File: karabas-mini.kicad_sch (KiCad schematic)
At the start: 4 parts

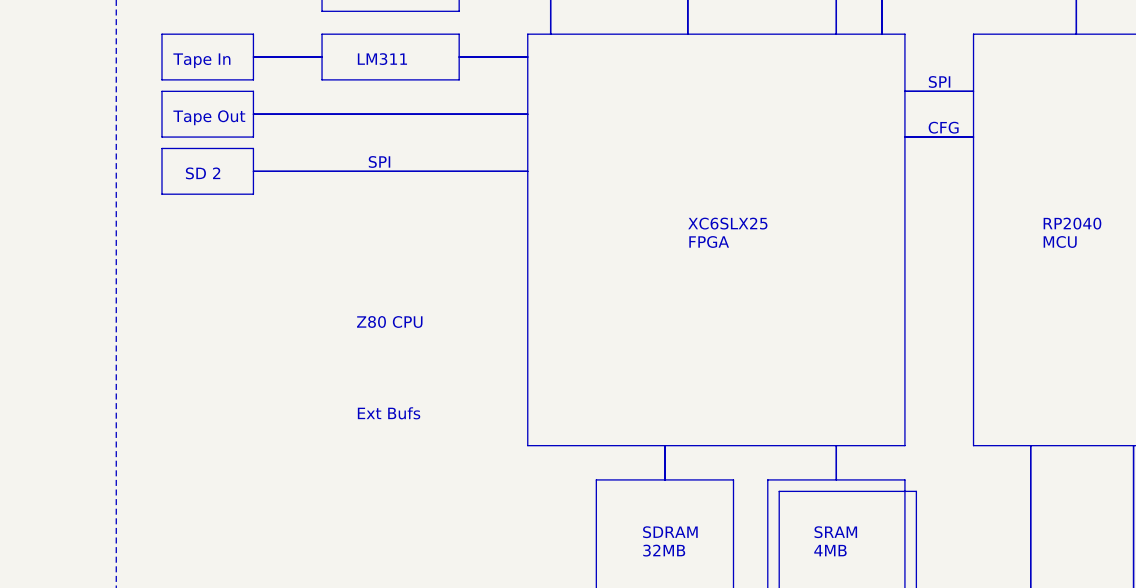
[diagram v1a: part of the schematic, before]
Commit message: Updated revB
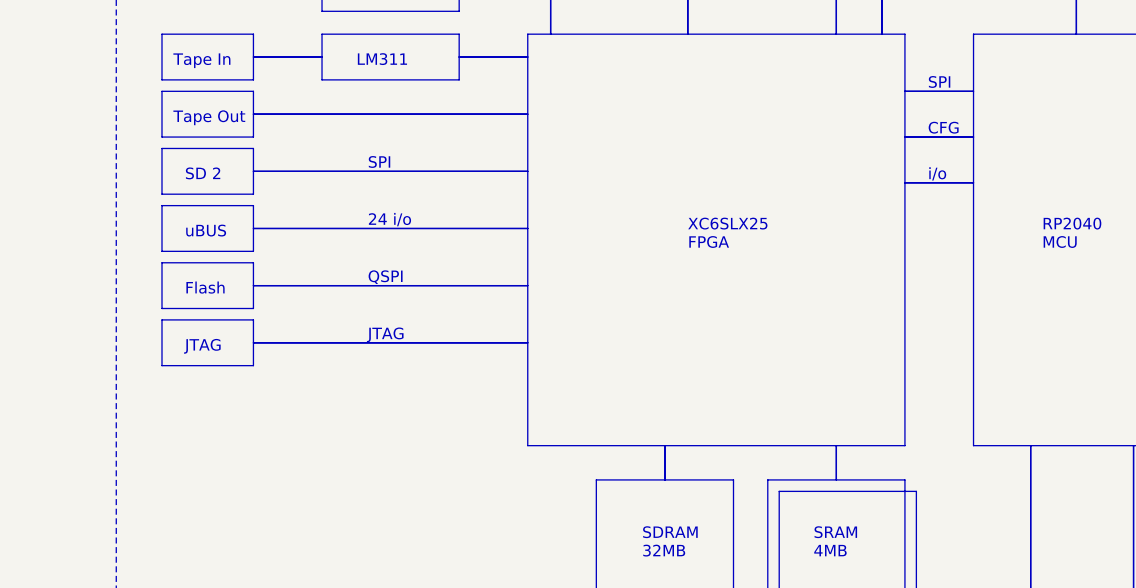
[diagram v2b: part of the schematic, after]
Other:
- note added: "24 i/o"
- note added: "JTAG"
- note added: "i/o"
- note added: "uBUS"
- note removed: "Ext Bufs"
- note removed: "Z80 CPU"
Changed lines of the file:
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@@
   (title_block
     (title "Karabas-Mini")
-    (date "2024-02-20")
-    (rev "A")
+    (date "2024-02-23")
+    (rev "B")
   )
   (rectangle (start 254 132.08) (end 264.16 137.16)
@@
     (fill (type none))
   )
+  (rectangle (start 194.31 91.44) (end 201.93 91.44)
+    (stroke (width 0) (type default))
+    (fill (type none))
+  )
   (rectangle (start 162.56 66.04) (end 177.8 71.12)
     (stroke (width 0) (type default))
@@
     (fill (type none))
   )
+  (rectangle (start 121.92 96.52) (end 152.4 96.52)
+    (stroke (width 0) (type default))
+    (fill (type none))
+  )
   (rectangle (start 144.78 69.85) (end 154.94 69.85)
     (stroke (width 0) (type default))
@@
     (fill (type none))
   )
+  (rectangle (start 111.76 106.68) (end 121.92 111.76)
+    (stroke (width 0) (type default))
+    (fill (type color) (color 255 255 194 1))
+  )
+  (rectangle (start 111.76 100.33) (end 121.92 105.41)
+    (stroke (width 0) (type default))
+    (fill (type color) (color 255 255 194 1))
+  )
   (rectangle (start 208.28 120.65) (end 208.28 138.43)
     (stroke (width 0) (type default))
@@
     (fill (type color) (color 255 255 194 1))
   )
+  (rectangle (start 121.92 102.87) (end 152.4 102.87)
+    (stroke (width 0) (type default))
+    (fill (type none))
+  )
   (rectangle (start 121.92 77.47) (end 129.54 77.47)
     (stroke (width 0) (type default))
@@
     (stroke (width 0) (type default))
     (fill (type none))
+  )
+  (rectangle (start 111.76 93.98) (end 121.92 99.06)
+    (stroke (width 0) (type default))
+    (fill (type color) (color 255 255 194 1))
   )
   (rectangle (start 226.06 81.28) (end 232.41 81.28)
@@
     (fill (type none))
   )
+  (rectangle (start 121.92 109.22) (end 152.4 109.22)
+    (stroke (width 0) (type default))
+    (fill (type none))
+  )
   (rectangle (start 33.02 34.29) (end 87.63 149.86)
     (stroke (width 0) (type dash))
@@
     (effects (font (size 1.27 1.27)) (justify left bottom))
   )
+  (text "24 i/o" (at 134.62 96.52 0)
+    (effects (font (size 1.27 1.27)) (justify left bottom))
+  )
+  (text "Flash" (at 114.3 104.14 0)
+    (effects (font (size 1.27 1.27)) (justify left bottom))
+  )
+  (text "i/o" (at 196.85 91.44 0)
+    (effects (font (size 1.27 1.27)) (justify left bottom))
+  )
   (text "XC6SLX25\nFPGA" (at 170.18 99.06 0)
     (effects (font (size 1.27 1.27)) (justify left bottom))
@@
     (effects (font (size 1.27 1.27)) (justify left bottom))
   )
-  (text "Z80 CPU" (at 133.35 107.95 0)
-    (effects (font (size 1.27 1.27) (color 255 255 255 1)) (justify left bottom))
-  )
   (text "SPI" (at 227.33 115.57 0)
     (effects (font (size 1.27 1.27)) (justify left bottom))
@@
     (effects (font (size 1.27 1.27)) (justify left bottom))
   )
-  (text "Ext Bufs" (at 133.35 118.11 0)
-    (effects (font (size 1.27 1.27) (color 255 255 255 1)) (justify left bottom))
-  )
   (text "SRAM\n4MB" (at 184.15 133.35 0)
     (effects (font (size 1.27 1.27)) (justify left bottom))
@@
     (effects (font (size 1.27 1.27)) (justify left bottom))
   )
+  (text "QSPI" (at 134.62 102.87 0)
+    (effects (font (size 1.27 1.27)) (justify left bottom))
+  )
   (text "Functional schematics" (at 109.22 39.37 0)
     (effects (font (size 1.27 1.27)) (justify left bottom))
@@
     (effects (font (size 1.27 1.27)) (justify left bottom))
   )
+  (text "uBUS" (at 114.3 97.79 0)
+    (effects (font (size 1.27 1.27)) (justify left bottom))
+  )
   (text "CFG" (at 196.85 86.36 0)
     (effects (font (size 1.27 1.27)) (justify left bottom))
@@
     (effects (font (size 1.27 1.27)) (justify left bottom))
   )
+  (text "JTAG" (at 134.62 109.22 0)
+    (effects (font (size 1.27 1.27)) (justify left bottom))
+  )
   (text "USB C" (at 256.54 72.39 0)
     (effects (font (size 1.27 1.27)) (justify left bottom))
@@
     (effects (font (size 1.27 1.27)) (justify left bottom))
   )
+  (text "JTAG" (at 114.3 110.49 0)
+    (effects (font (size 1.27 1.27)) (justify left bottom))
+  )

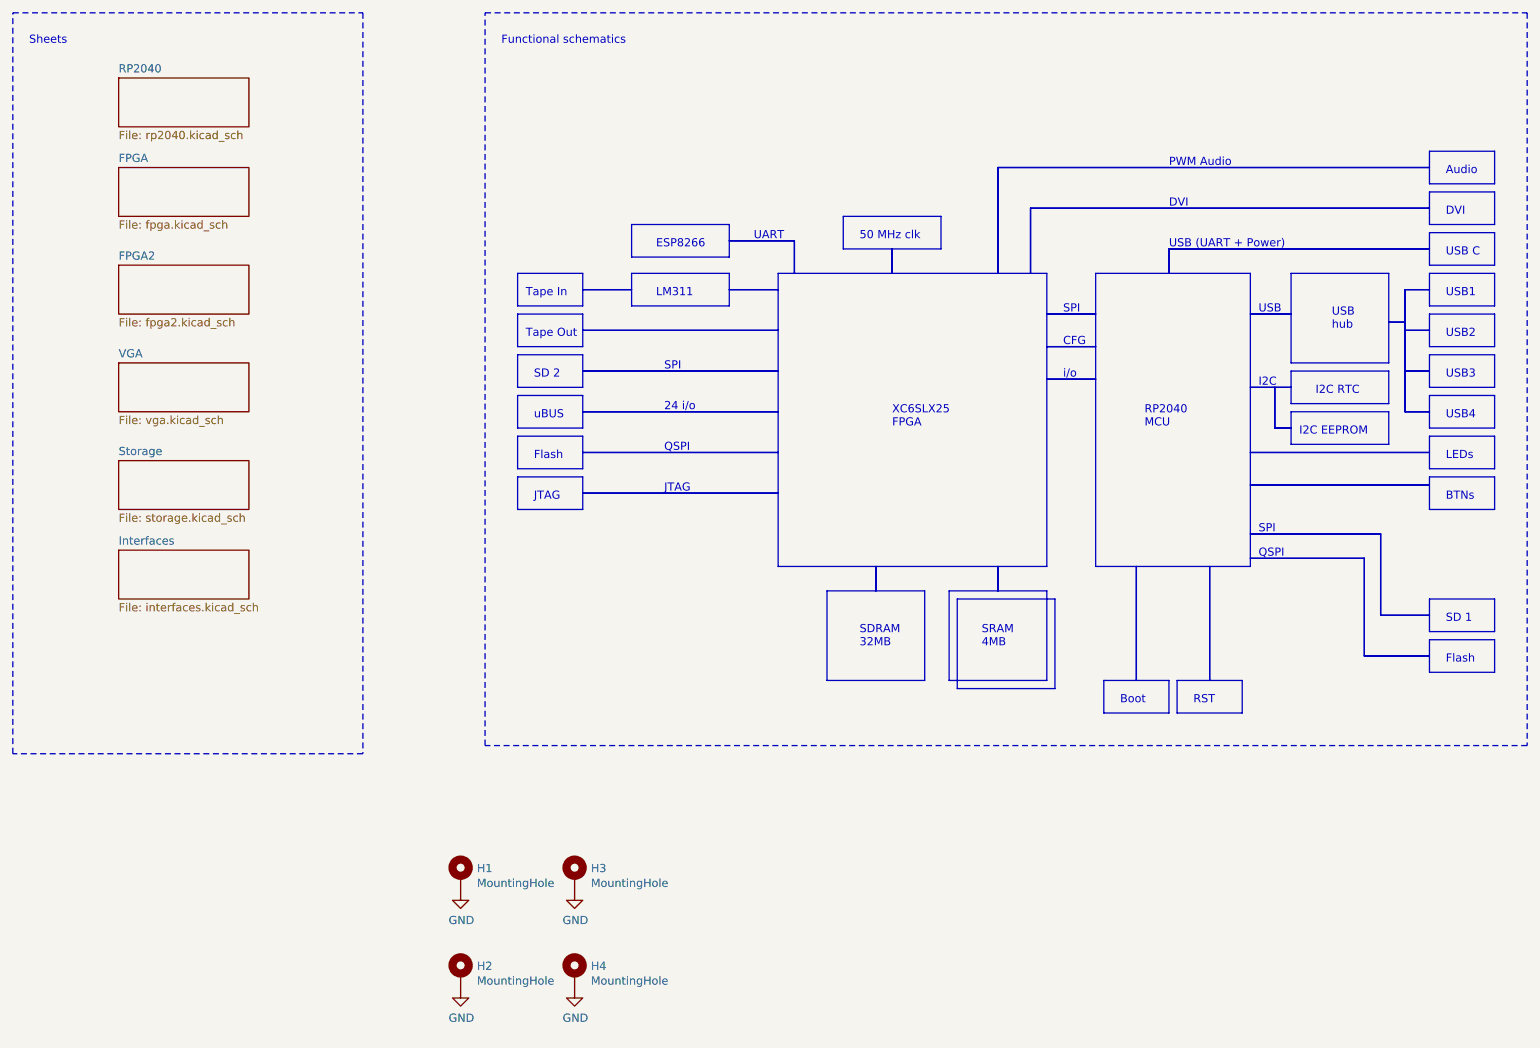
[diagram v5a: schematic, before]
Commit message: revG
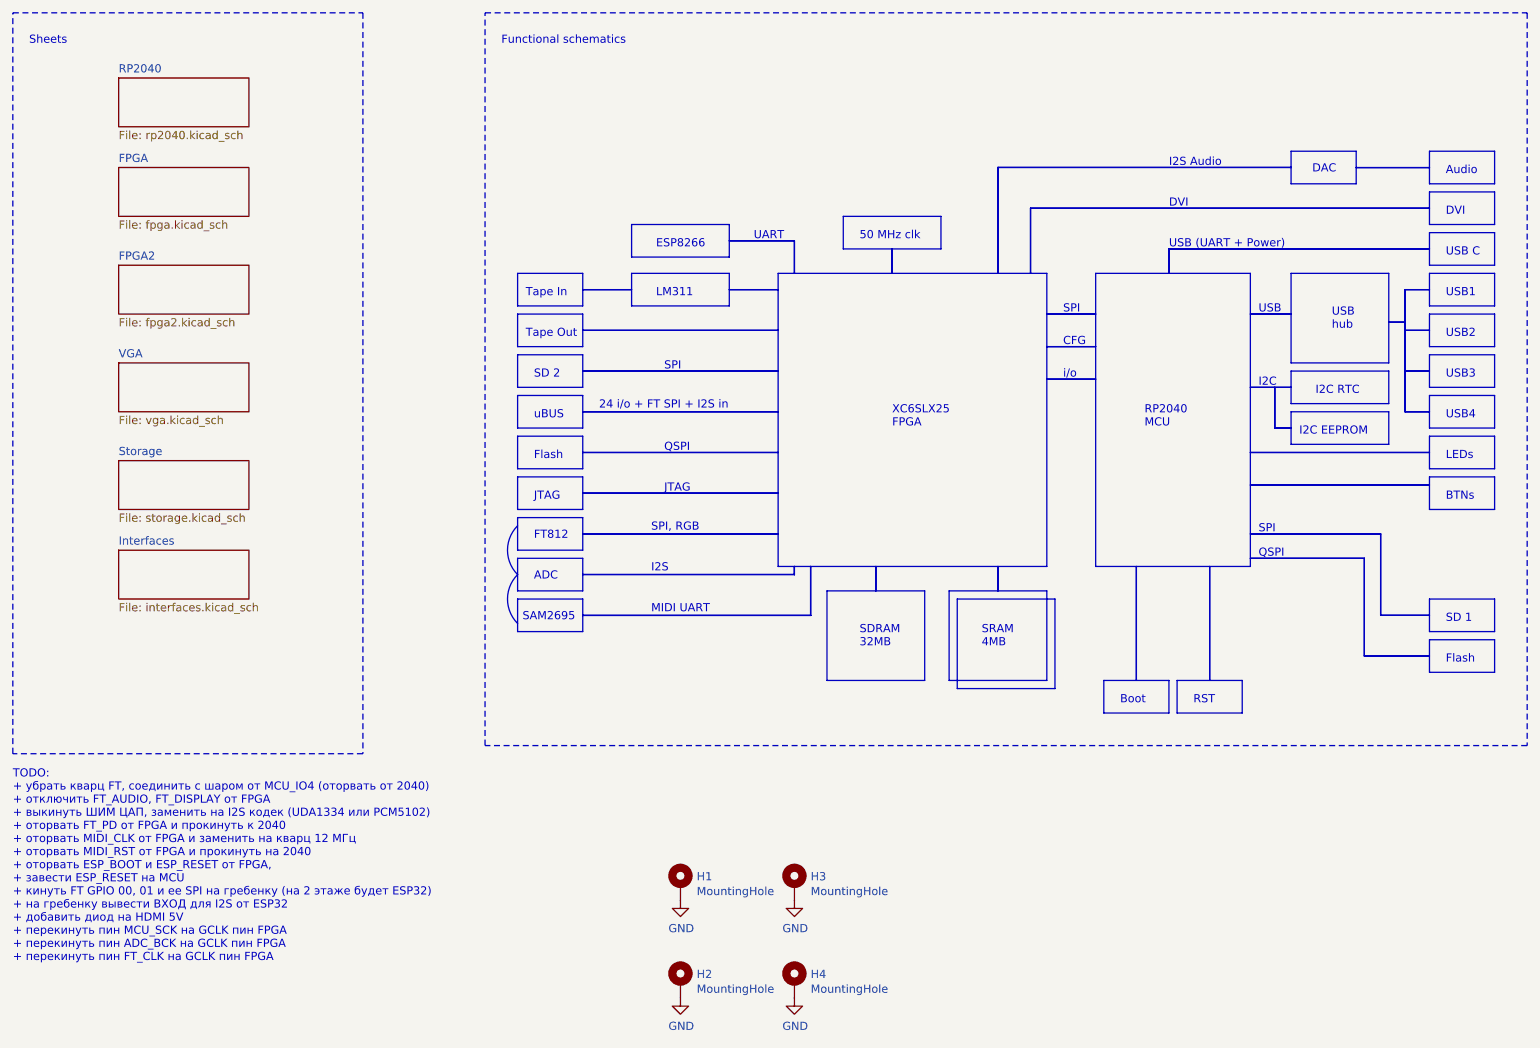
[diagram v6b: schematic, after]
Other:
- note added: "24 i/o + FT SPI + I2S in"
- note added: "ADC"
- note added: "DAC"
- note added: "FT812"
- note added: "I2S"
- note added: "I2S Audio"
- note added: "MIDI UART"
- note added: "SAM2695"
- note added: "SPI, RGB"
- note added: "TODO: + убрать кварц FT, соединить с шаром от MCU_IO4 (оторвать от 2040) + отключить FT_AUDIO, FT_DISPLAY от FPGA + выкинуть ШИМ ЦАП, заменить на I2S кодек (UDA1334 или PCM5102) + оторвать FT_PD от FPGA и прокинуть к 2040 + оторвать MIDI_CLK от FPGA и заменить на кварц 12 МГц + оторвать MIDI_RST от FPGA и прокинуть на 2040 + оторвать ESP_BOOT и ESP_RESET от FPGA, + завести ESP_RESET на MCU + кину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"
- note removed: "24 i/o"
- note removed: "PWM Audio"
- moved on the sheet: H1, H2, H3, H4
